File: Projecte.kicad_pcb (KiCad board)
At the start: 2 copper layers, 69.3 x 53.3 mm, 76 parts, among them K1 A161CS12VDC.64, Q1 IRLZ34N, Q3 IRLZ34N, Q4 IRLZ34N, Q5 IRLZ34N, Q7 IRLZ34N, U1 PIC18F448-IP, U2 OPA336Nx, U3 LM1117DT-5.0, U4 MCP2551-I-P, U5 AMS1117-3.3, U6 PCA9306, U7 TPS63070RNMR, U8 MMC5883MA, Y1 Crystal

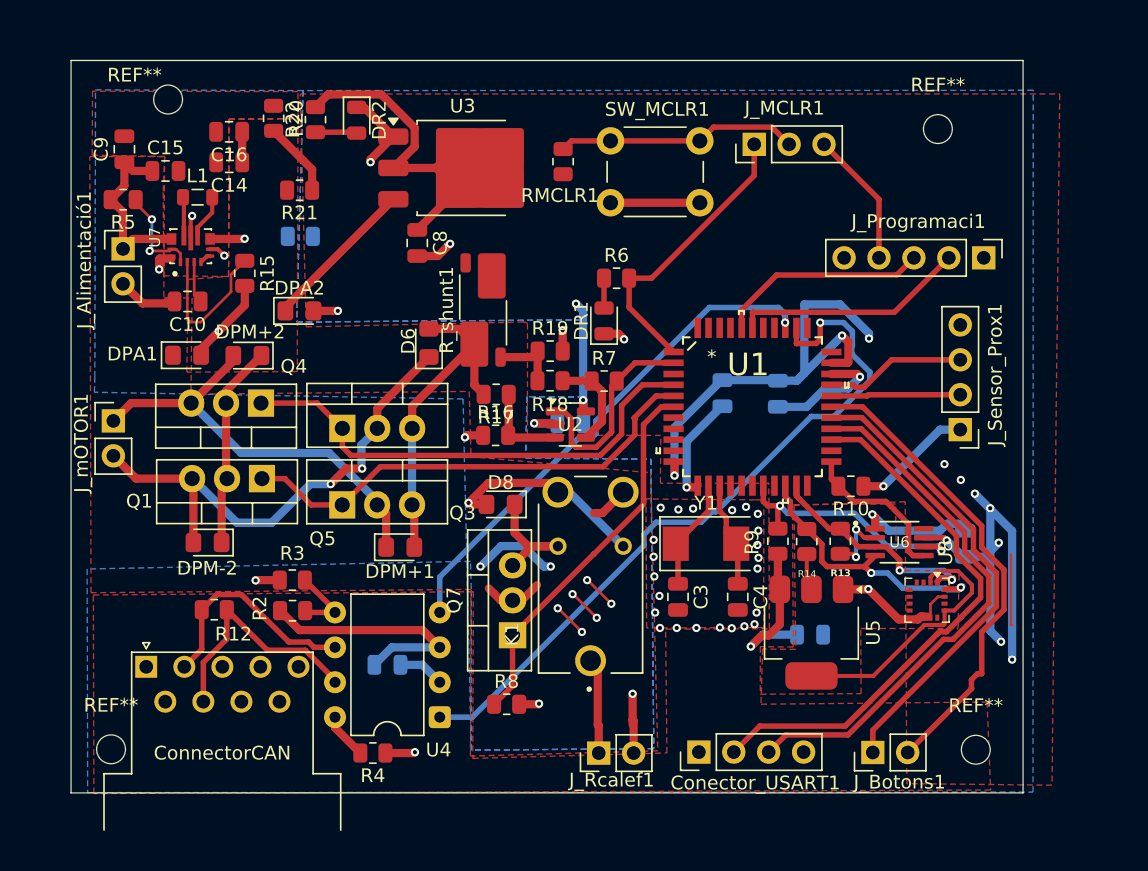
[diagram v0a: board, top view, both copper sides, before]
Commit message: Layout_Final
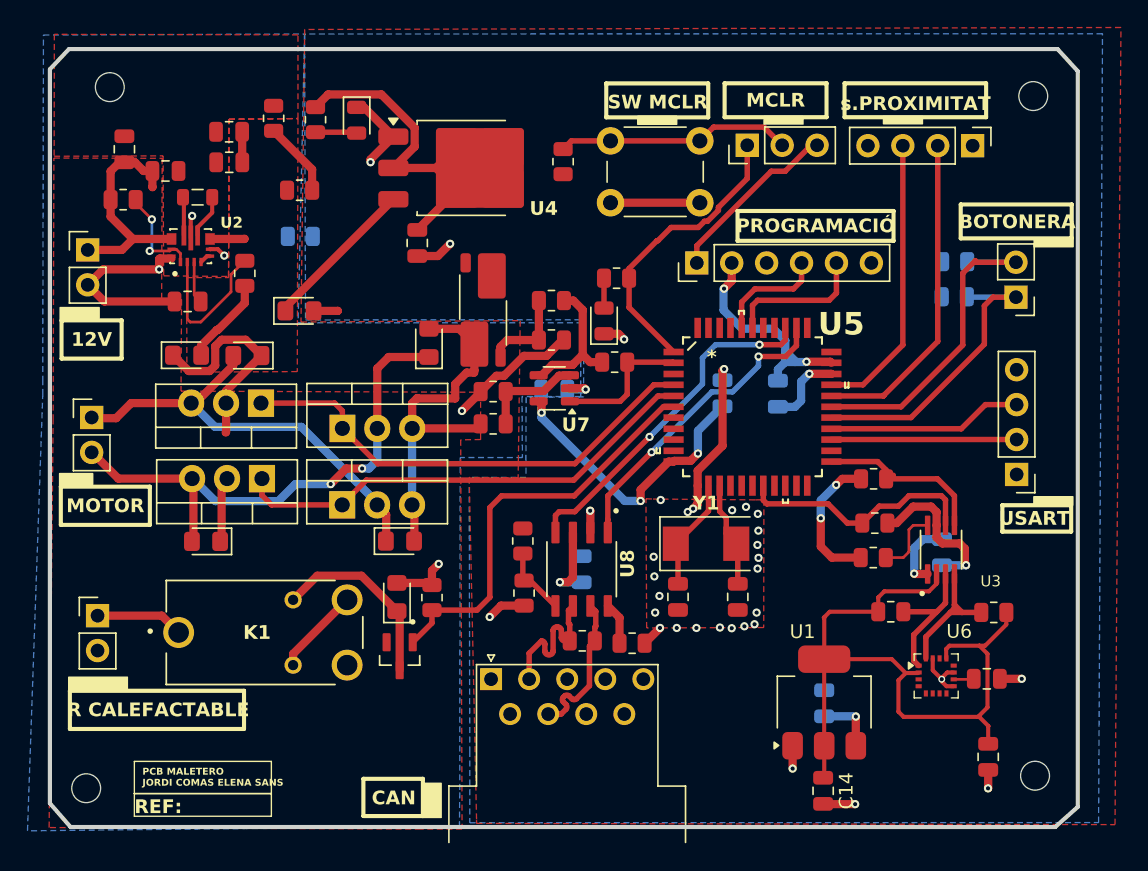
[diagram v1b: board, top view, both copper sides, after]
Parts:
- removed J_Programaci1: Conn_01x05_Pin, Connector_PinHeader_2.54mm:PinHeader_1x05_P2.54mm_Vertical
- removed the R10 at (214.8, 105.0)
- removed the R13 at (214.0, 109.0)
- removed the R14 at (211.6, 109.0)
- removed the R9 at (209.4, 109.0)
- removed the U5 at (211.9, 115.6)
- removed the U8 at (220.3, 113.3)
- added C13: 10u, Capacitor_SMD:C_0805_2012Metric, F.Cu at (224.7, 119.0)
- added C14: 1u, Capacitor_SMD:C_0805_2012Metric, F.Cu at (212.7, 127.1)
- added C2: 22u, Capacitor_SMD:C_0805_2012Metric, F.Cu at (224.8, 124.7)
- added PROGRAMACIÓ: Conn_01x06_Pin, Connector_PinHeader_2.54mm:PinHeader_1x06_P2.54mm_Vertical, F.Cu at (203.6, 88.7)
- added R12: 2.7k, Resistor_SMD:R_0805_2012Metric, F.Cu at (216.4, 104.4)
- added R23: 200k, Resistor_SMD:R_0805_2012Metric, B.Cu at (222.3, 91.2)
- added R24: 200k, Resistor_SMD:R_0805_2012Metric, B.Cu at (222.3, 88.6)
- added R3: 2.7k, Resistor_SMD:R_0805_2012Metric, F.Cu at (225.2, 114.2)
- added R5: 2.7k, Resistor_SMD:R_0805_2012Metric, F.Cu at (217.7, 114.1)
- added R6: 200k, Resistor_SMD:R_0805_2012Metric, F.Cu at (216.4, 110.2)
- added R7: 2.7k, Resistor_SMD:R_0805_2012Metric, F.Cu at (216.5, 107.7)
- added U1: AMS1117-3.3, Package_TO_SOT_SMD:SOT-223-3_TabPin2, F.Cu at (212.8, 120.7)
- added U3: PCA9306, Library:PCA, F.Cu at (221.3, 109.6)
- Q1: renamed from Q7; footprint Package_TO_SOT_THT:TO-220-3_Vertical -> Library:SOT95P237X112-3N
- R CALEFACTABLE: renamed from J_Rcalef1
- SW MCLR: renamed from SW_MCLR1
- U6: value PCA9306 -> MMC5883MA; footprint Library:PCA -> Package_LGA:LGA-16_3x3mm_P0.5mm
- U8: renamed from U4; footprint Package_DIP:DIP-8_W7.62mm -> Library:SOIC127P599X175-8N
- moved R CALEFACTABLE 37.8 mm to (159.9, 114.4), turned to 0 degrees
- moved BOTONERA 34.7 mm to (226.8, 91.2), turned to 180 degrees
- moved USART 30.7 mm to (226.8, 104.1), turned to 180 degrees
- moved R22 26.9 mm to (195.2, 116.2)
- moved CAN 25.1 mm to (188.6, 119.0)
- moved K1 24.1 mm to (172.1, 115.6), turned to 0 degrees
- moved s.PROXIMITAT 20.7 mm to (223.6, 80.2), turned to -90 degrees
- moved R17 20.5 mm to (198.8, 116.4)
- moved R19 17.5 mm to (190.9, 109.0), turned to -90 degrees
- moved R21 16.9 mm to (191.0, 112.7), turned to -90 degrees
- moved C11 15.7 mm to (195.2, 111.0), turned to 90 degrees
- moved U8 14.9 mm to (195.2, 111.0), turned to -90 degrees
- moved D1 10.1 mm to (181.7, 113.0), turned to 90 degrees
- moved U6 10.1 mm to (221.0, 118.8)
- moved R13 9.47 mm to (184.3, 113.1), turned to 90 degrees
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- renumbered J_Alimentació1 to 12V, J_Botons1 to BOTONERA, C14 to C10, C16 to C11, C8 to C12, C17 to C15, C5 to C16, C9 to C4, C4 to C5, C10 to C6, C15 to C7, C7 to C8, C6 to C9, ConnectorCAN to CAN, D8 to D1, D6 to D2, DPM+2 to DPM+1, DPM+1 to DPM+2, DPM-2 to DPM-1, J_MCLR1 to MCLR, J_mOTOR1 to MOTOR, Q4 to Q2, Q5 to Q3, Q1 to Q4, Q3 to Q5, R11 to R1, R22 to R10, R15 to R11, R8 to R13, R19 to R14, R17 to R15, R18 to R16, R4 to R17, R16 to R18, R2 to R19, R6 to R2, R7 to R20, R3 to R21, R12 to R22, R5 to R4, R21 to R8, R20 to R9, U7 to U2, U3 to U4, U1 to U5, U2 to U7, Conector_USART1 to USART, J_Sensor_Prox1 to s.PROXIMITAT
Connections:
- U5 pad 20: /SDA_S -> unconnected-(U5-C1IN-/PSP1/RD1-Pad20)
- U5 pad 21: /SCL_S -> unconnected-(U5-C2IN+/PSP2/RD2-Pad21)
- U6 pad 1: GND -> /SCL_S
- U6 pad 3: /SCL_S -> unconnected-(U6-NC-Pad3)
- U6 pad 4: /SDA_S -> unconnected-(U6-NC-Pad4)
- U6 pad 5: /SDA -> unconnected-(U6-NC-Pad5)
- U6 pad 6: /SCL -> unconnected-(U6-NC-Pad6)
- U6 pad 7: VCC -> unconnected-(U6-NC-Pad7)
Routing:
- net VCC: track 156.0 -> 109.9 mm, vias 16 -> 10
- net /Tx: track 52.9 -> 22.6 mm, vias 1 -> 2
- net /usart_tx: track 39.8 -> 13.5 mm
- net /Vcc_3.3V: track 27.0 -> 53.2 mm, vias 2 -> 0
- net /usart_rx: track 39.2 -> 14.2 mm
- net /S_entrada: track 9.42 -> 23.6 mm
- net /Rx: track 37.6 -> 25.3 mm, vias 1 -> 2
- net /Boto_Motor: track 34.4 -> 22.3 mm
- net /S_sortida: track 10.3 -> 20.9 mm
- net /Boto_R: track 34.8 -> 24.5 mm
- net /SDA_S: track 20.2 -> 10.0 mm, vias 2 -> 0
- net /PGD: track 15.4 -> 8.17 mm
- net /PGC: track 17.1 -> 10.3 mm
- net /SCL_S: track 16.8 -> 10.2 mm, vias 2 -> 0
- net /Canh: track 17.6 -> 11.1 mm
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- removed copper zone on F.Cu, net /Vcc_3.3V
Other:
- board size 69.3 x 53.3 mm -> 74.8 x 56.6 mm
- board text added: "PCB MALETERO JORDI COMAS ELENA SANS"
- board text added: "REF:"

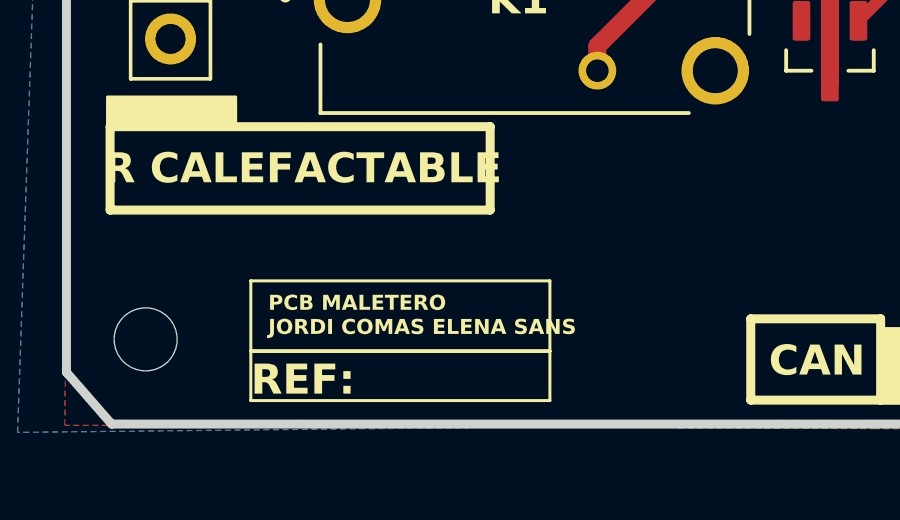
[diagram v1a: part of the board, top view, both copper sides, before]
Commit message: .
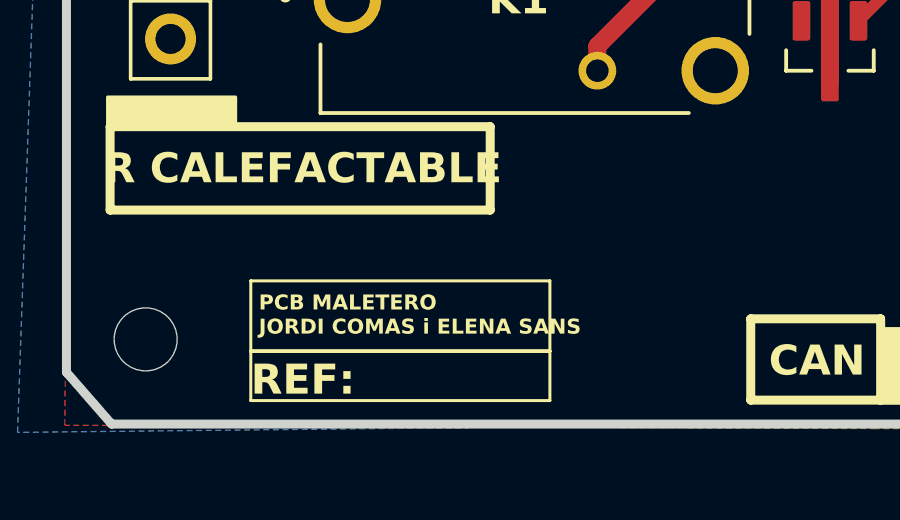
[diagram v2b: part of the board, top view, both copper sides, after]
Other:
- board text added: "PCB MALETERO JORDI COMAS i ELENA SANS"
- board text removed: "PCB MALETERO JORDI COMAS ELENA SANS"
